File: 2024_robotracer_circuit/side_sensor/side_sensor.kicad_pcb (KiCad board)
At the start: 2 copper layers, 9 parts, among them J2 PH_5p, U1 LBR-127HLD

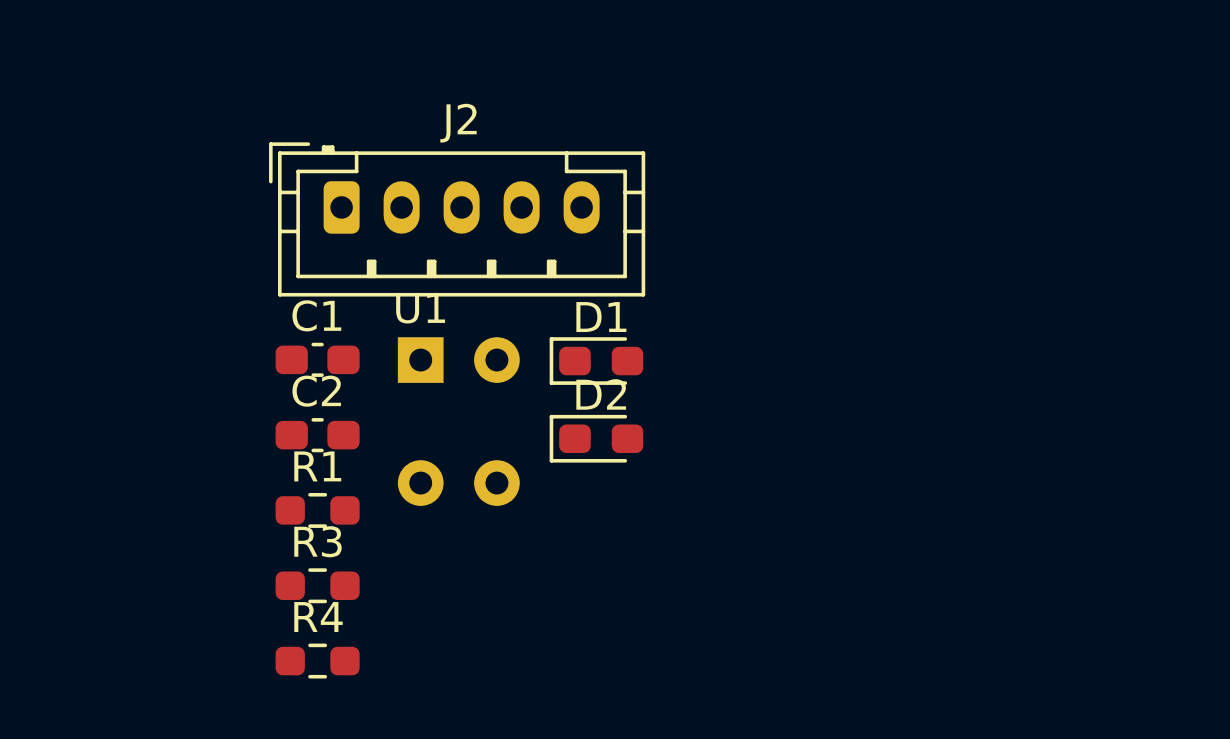
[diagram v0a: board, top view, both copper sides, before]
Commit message: サイドセンサ
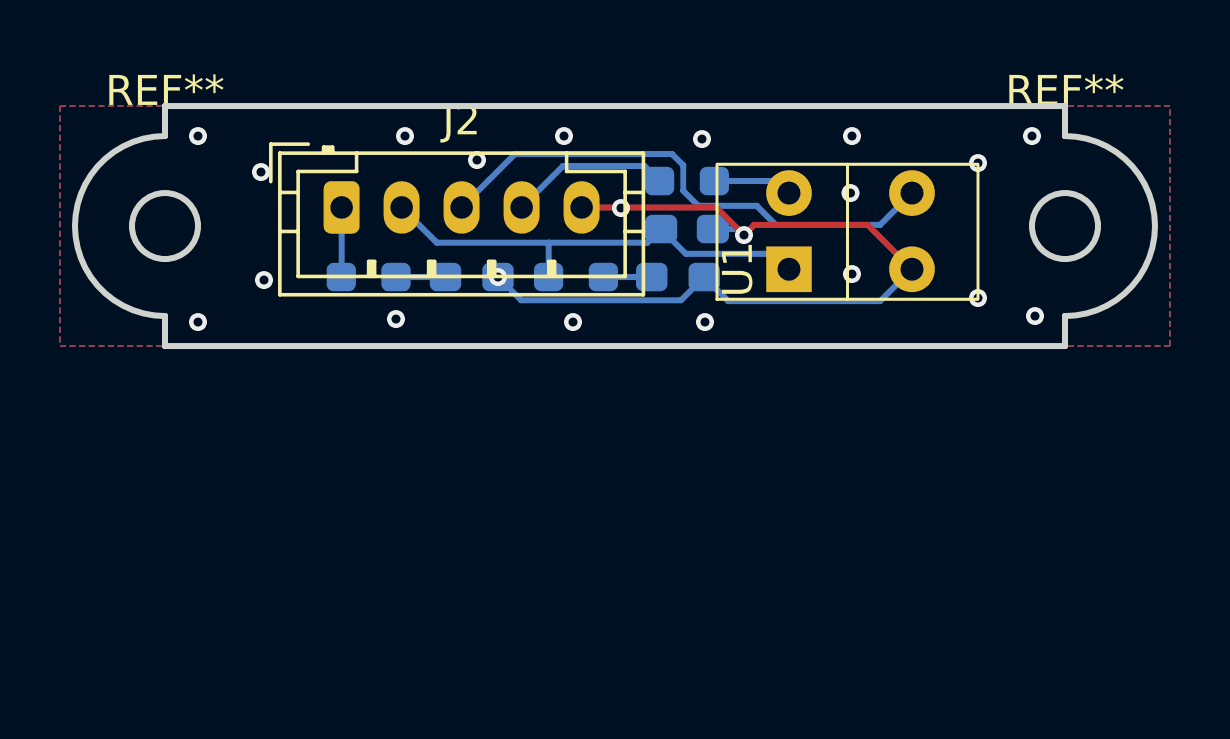
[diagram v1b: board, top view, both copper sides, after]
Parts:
- removed C1: 0.1u, Capacitor_SMD:C_0603_1608Metric_Pad1.08x0.95mm_HandSolder
- added REF**: MountingHole_2.2mm_M2, MountingHole:MountingHole_2.2mm_M2, F.Cu at (144.5, 87.0)
- added REF**: MountingHole_2.2mm_M2, MountingHole:MountingHole_2.2mm_M2, F.Cu at (174.5, 87.0)
- C2, D1, D2, R1, R3, R4: moved to B.Cu
- moved R1 16.5 mm to (161.9, 85.5), turned to 180 degrees
- moved R4 15.4 mm to (158.2, 88.7)
- moved C2 14.1 mm to (161.9, 87.1)
- moved U1 12.6 mm to (165.3, 88.4), turned to 90 degrees
- moved R3 10.4 mm to (151.3, 88.7)
- moved D2 5.97 mm to (161.6, 88.7), turned to 180 degrees
- moved D1 5.15 mm to (154.7, 88.7), turned to 180 degrees
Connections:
- U1 pad 4: /SENSOR0_ADC -> /SENSOR_SIDE_ADC
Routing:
- net GND: track 0.00 -> 28.5 mm, vias 0 -> 21
- net /SENSOR_SIDE_ADC: track 0.00 -> 17.7 mm
- net +5V: track 0.00 -> 15.3 mm
- net /PULSE: track 0.00 -> 5.38 mm
- net Net-(U1-cathode): track 0.00 -> 2.65 mm
- net +3.3V: track 0.00 -> 2.33 mm
- net Net-(D1-A): track 0.00 -> 1.65 mm
- net Net-(D2-A): track 0.00 -> 1.61 mm
- added copper zone on B.Cu, net GND
- added copper zone on F.Cu, net GND
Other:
- board outline added: 36 x 8 mm

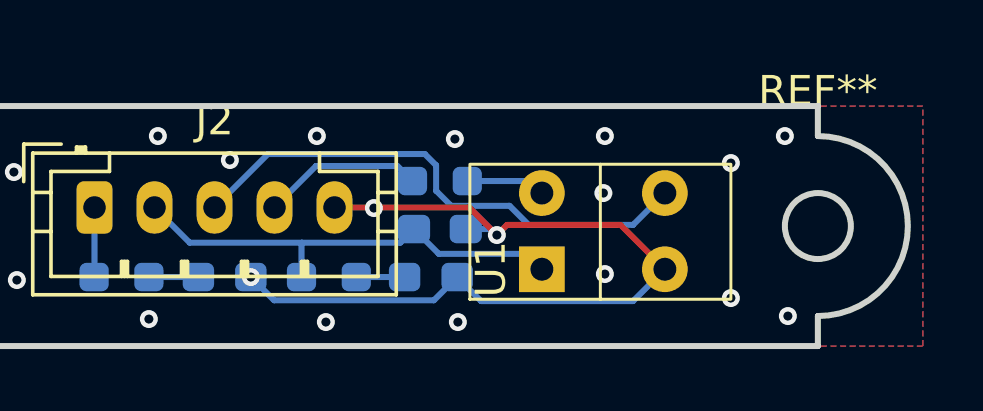
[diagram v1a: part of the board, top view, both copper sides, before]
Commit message: 修正
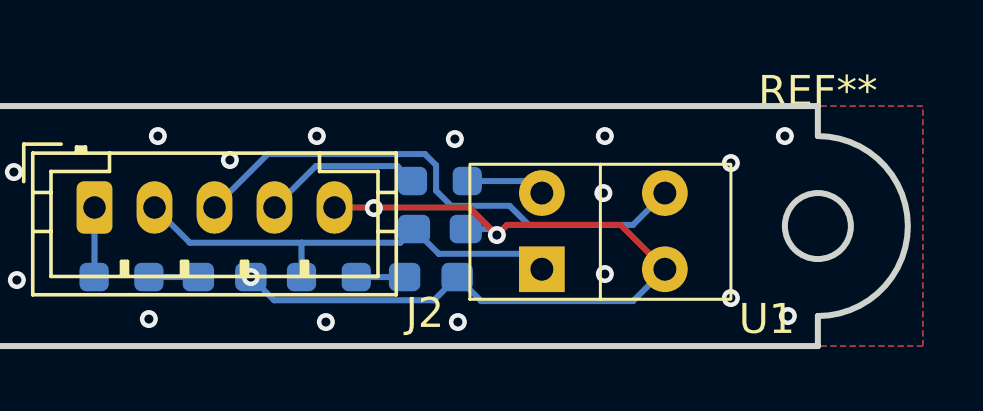
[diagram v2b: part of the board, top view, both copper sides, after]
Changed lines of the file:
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@@
 		(tags "connector JST PH side entry")
 		(property "Reference" "J2"
-			(at 4 -2.9 0)
+			(at 11.0125 3.52 0)
 			(layer "F.SilkS")
 			(effects
@@
 		(at 165.3 88.44 90)
 		(property "Reference" "U1"
-			(at 0 -1.7 90)
+			(at -1.66 7.5 0)
 			(unlocked yes)
 			(layer "F.SilkS")
@@
 		(tags "resistor handsolder")
 		(property "Reference" "R1"
-			(at 0 1.43 180)
+			(at -2.2 1.2 180)
 			(layer "B.SilkS")
 			(effects
@@
 		(tags "capacitor handsolder")
 		(property "Reference" "C2"
-			(at 0 1.43 360)
+			(at 2.2 3 360)
 			(layer "B.SilkS")
 			(effects
@@
 		(tags "LED handsolder")
 		(property "Reference" "D1"
-			(at 0 1.43 180)
+			(at 0 -1.5 180)
 			(layer "B.SilkS")
 			(effects
@@
 		(tags "LED handsolder")
 		(property "Reference" "D2"
-			(at 0 1.43 180)
+			(at -2.5 1.5 180)
 			(layer "B.SilkS")
 			(effects
@@
 		(min_thickness 0.25)
 		(filled_areas_thickness no)
-		(fill yes
+		(fill
 			(thermal_gap 0.5)
 			(thermal_bridge_width 0.5)
